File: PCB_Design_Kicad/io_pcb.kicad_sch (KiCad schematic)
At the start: 14 parts, among them J17 MIDI in, J3 Voct_A, J4 Trig_A, J5 Vel_A, J6 Voct_B, J7 Trig_B, J8 Vel_B, J9 adv_clock_out, SW1 midi learn, SW2 re-sync, SW3 seq. mode

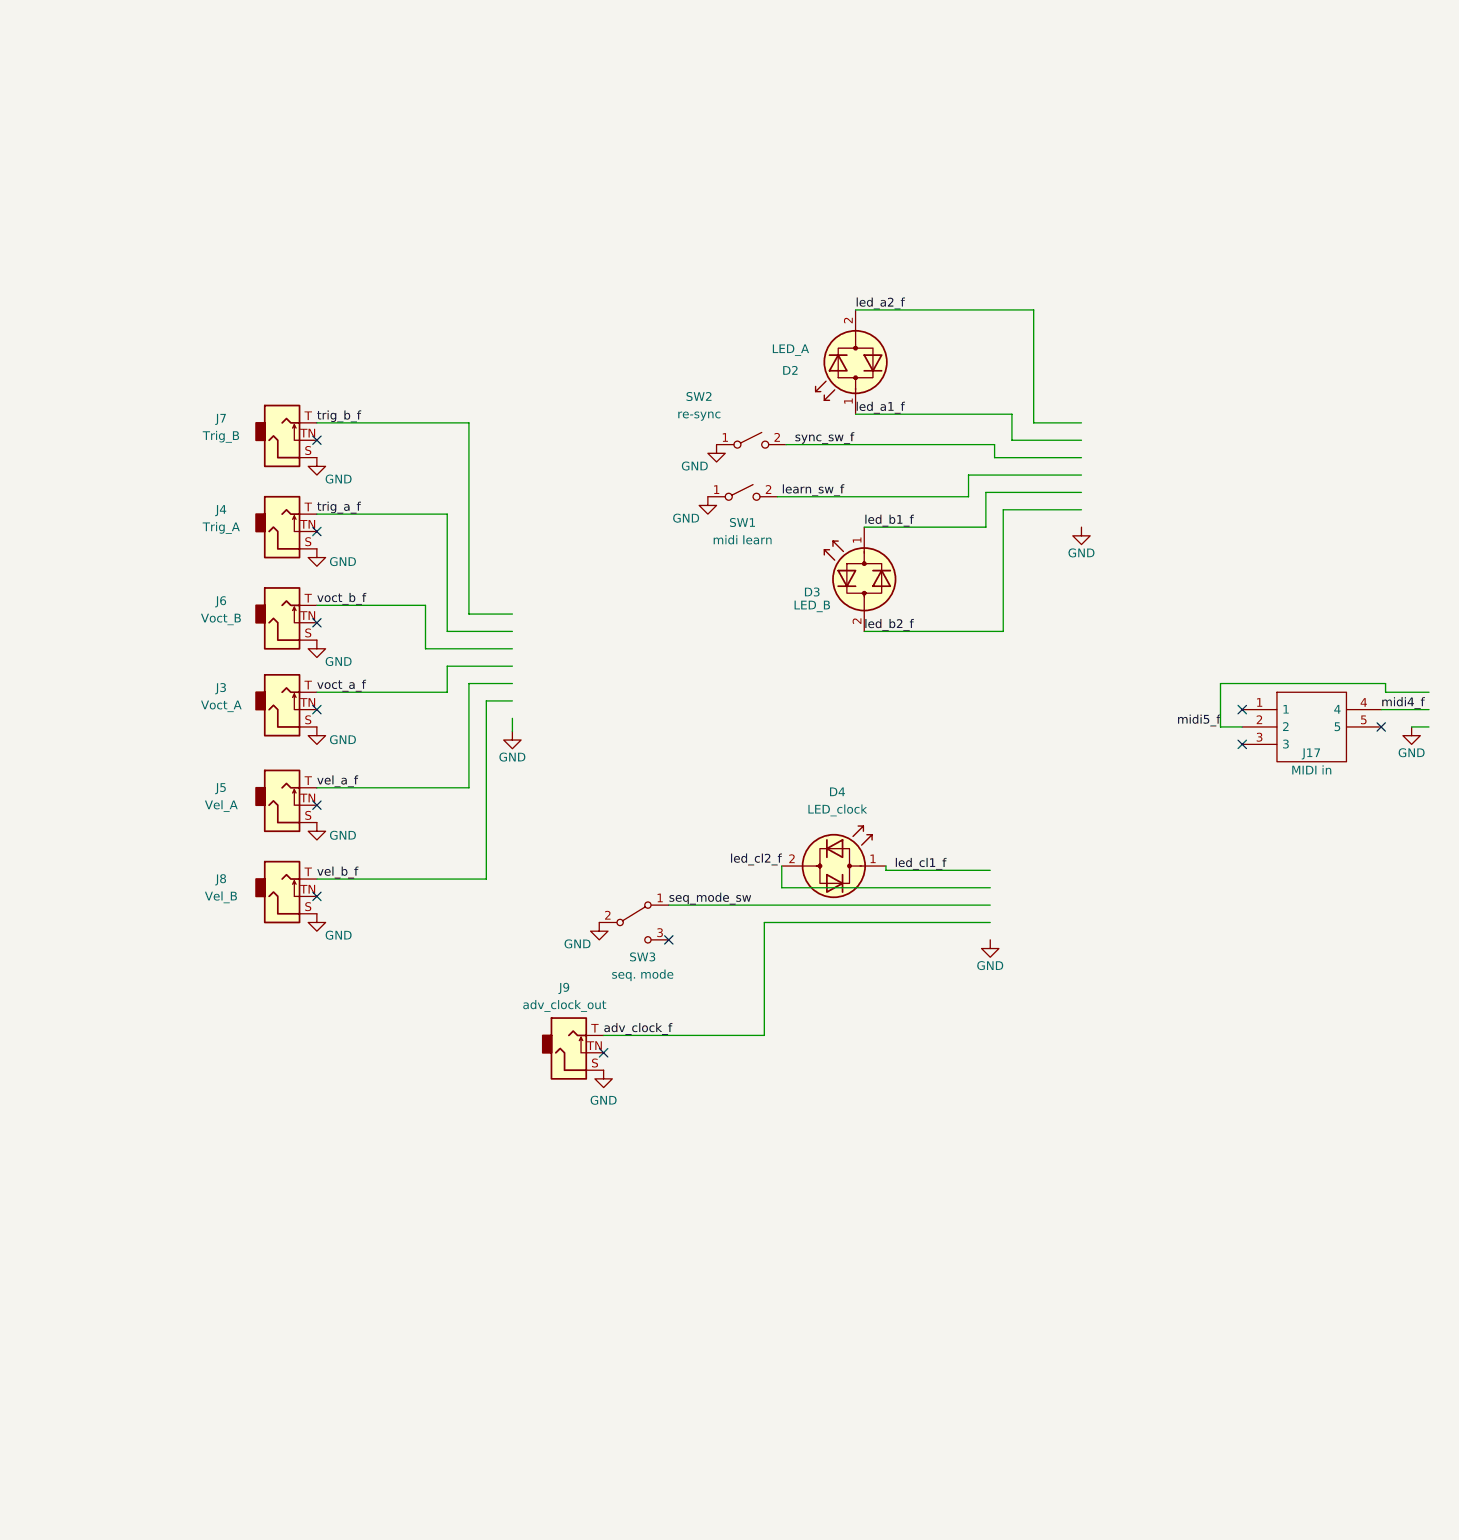
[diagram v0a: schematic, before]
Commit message: better routing
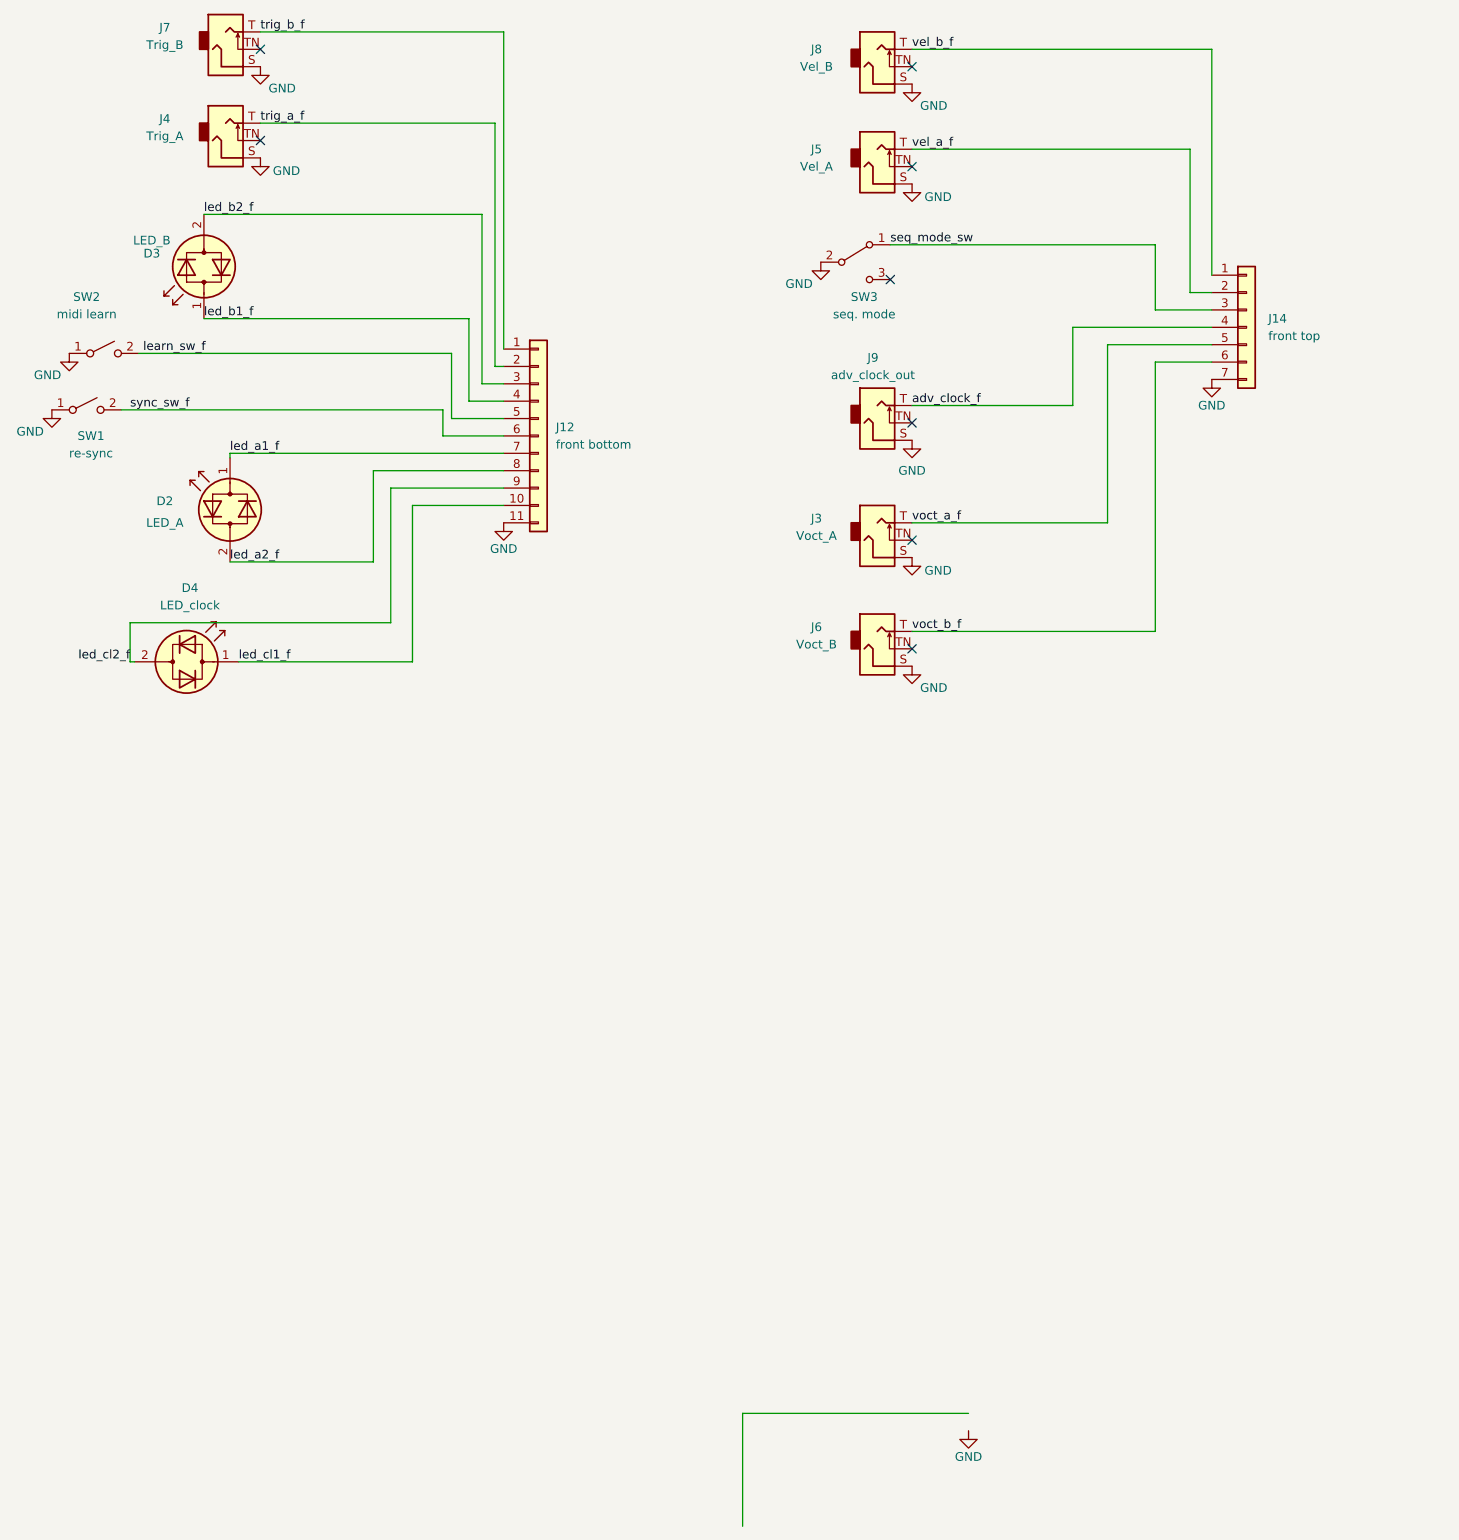
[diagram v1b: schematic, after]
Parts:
- removed J17: MIDI in, SamacSys_Parts:SD-50BV, symbol SamacSys_Parts:SD-50BV
- added J12: front bottom, Connector_PinSocket_2.54mm:PinSocket_1x11_P2.54mm_Vertical, symbol Connector_Generic:Conn_01x11
- added J14: front top, Connector_PinSocket_2.54mm:PinSocket_1x07_P2.54mm_Vertical, symbol Connector_Generic:Conn_01x07
- SW1: value midi learn -> re-sync
- SW2: value re-sync -> midi learn
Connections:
- net GND: now also J12.11 (Pin_11), J14.7 (Pin_7)
- net adv_clock_f: now also J14.4 (Pin_4)
- net learn_sw_f: now also SW2.2 (B), J12.5 (Pin_5); no longer SW1.2 (B)
- net led_a1_f: now also J12.7 (Pin_7)
- net led_a2_f: now also J12.8 (Pin_8)
- net led_b1_f: now also J12.4 (Pin_4)
- net led_b2_f: now also J12.3 (Pin_3)
- net led_cl1_f: now also J12.10 (Pin_10)
- net led_cl2_f: now also J12.9 (Pin_9)
- net seq_mode_sw: now also J14.3 (Pin_3)
- net sync_sw_f: now also SW1.2 (B), J12.6 (Pin_6); no longer SW2.2 (B)
- net trig_a_f: now also J12.2 (Pin_2)
- net trig_b_f: now also J12.1 (Pin_1)
- net vel_a_f: now also J14.2 (Pin_2)
- net vel_b_f: now also J14.1 (Pin_1)
- net voct_a_f: now also J14.5 (Pin_5)
- net voct_b_f: now also J14.6 (Pin_6)
- no-connect marks 11 -> 8
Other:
- moved on the sheet: D2, D4, J3, J4, J5, J6, J7, J8
